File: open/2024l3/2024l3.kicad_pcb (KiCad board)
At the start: 2 copper layers, 173.6 x 90 mm, 2 parts, among them U1 OpenMV, U2 xiao-esp32c3

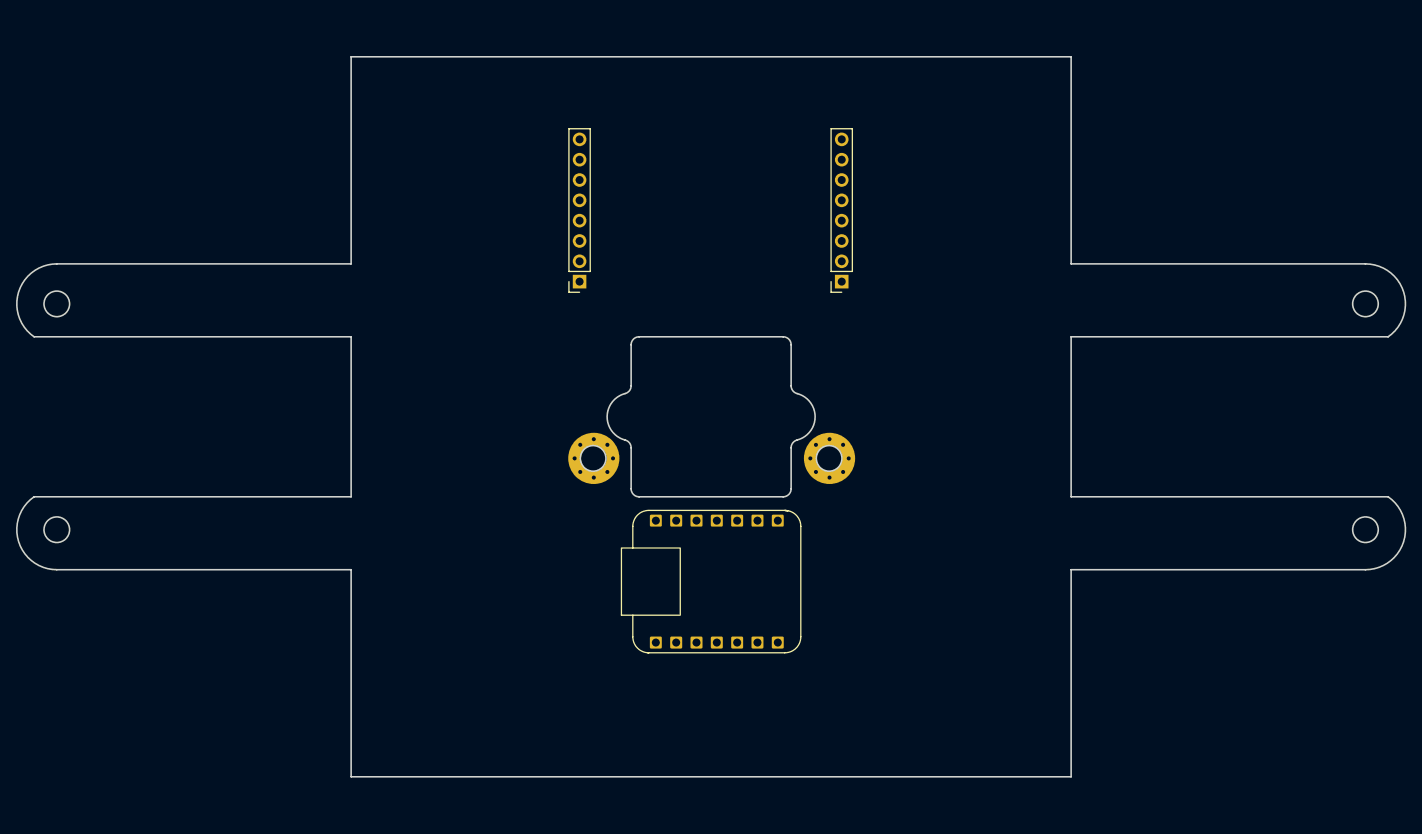
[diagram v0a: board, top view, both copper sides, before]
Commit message: open - l3 - 3d models
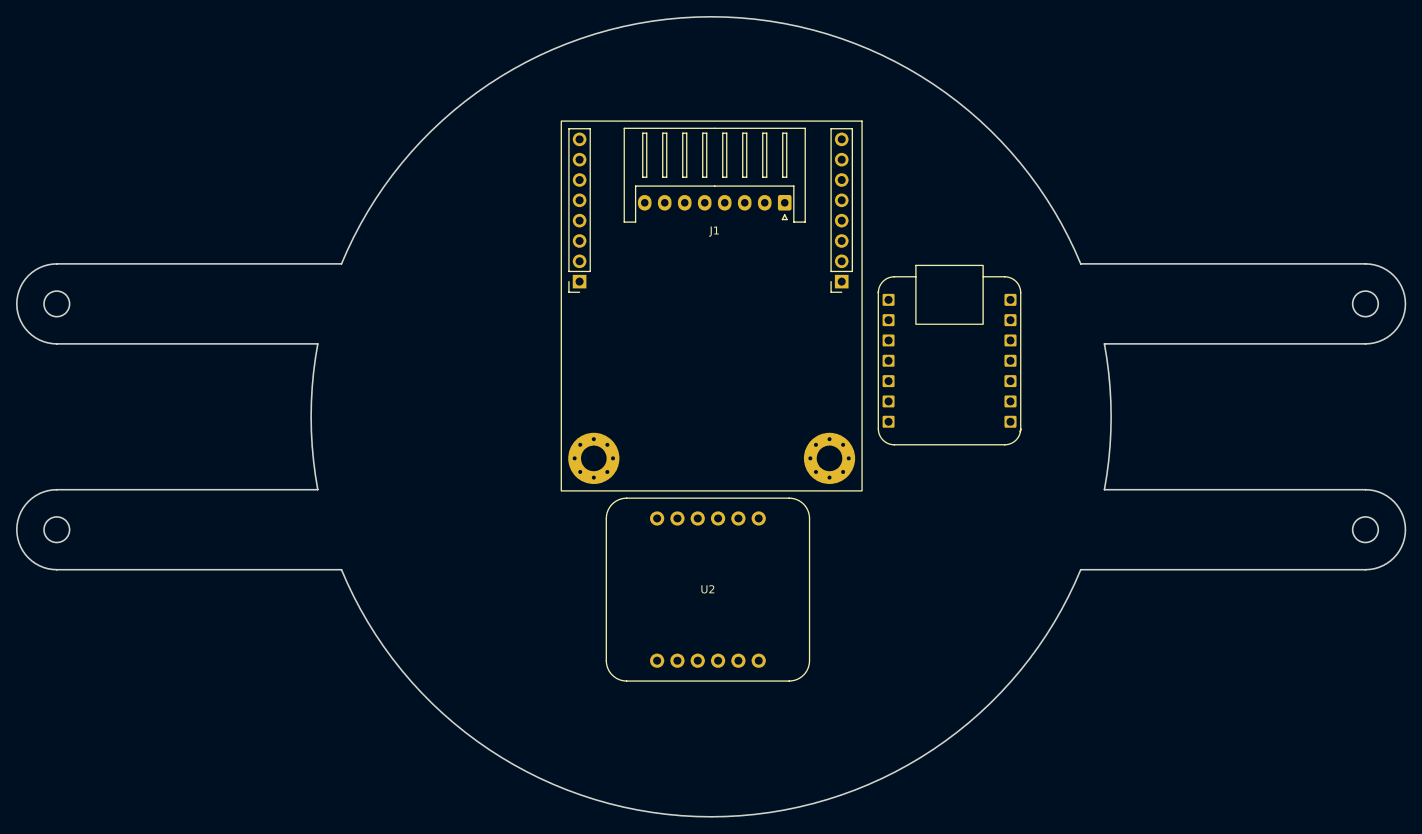
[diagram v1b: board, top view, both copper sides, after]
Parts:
- added J1: Conn_01x08, Connector_JST:JST_XH_S8B-XH-A_1x08_P2.50mm_Horizontal, F.Cu at (166.8, 79.6)
- added U3: xiao-esp32c3, 2024l3:xiao-esp32c3, F.Cu at (187.4, 99.3)
- U2: value xiao-esp32c3 -> 4754; footprint 2024l3:xiao-esp32c3 -> 2024l3:bno085
- moved U2 1.50 mm to (157.2, 127.9), turned to 180 degrees
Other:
- board size 173.6 x 90 mm -> 173.6 x 100 mm
